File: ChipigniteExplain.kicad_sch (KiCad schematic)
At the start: 73 parts, among them J1 Conn_01x02, J2 Conn_01x02, J3 Conn_01x03, J4 USB_C, J5 613012243121, J6 613012243121, J7 Conn_02x03_Odd_Even, Q1 DMN2005K, SW1 434121025816, SW2 434121025816, SW6 193-8MSR, U1 TLV1117LV33, U2 TPD1E05U06QDPYRQ1, U3 157112V12700

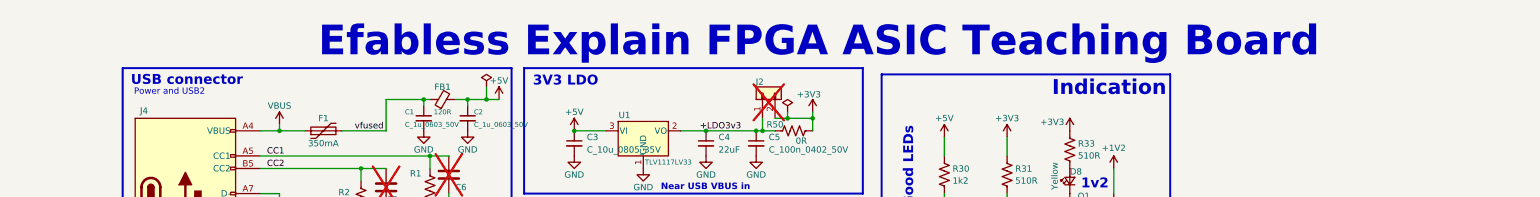
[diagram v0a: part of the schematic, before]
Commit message: title + attrib
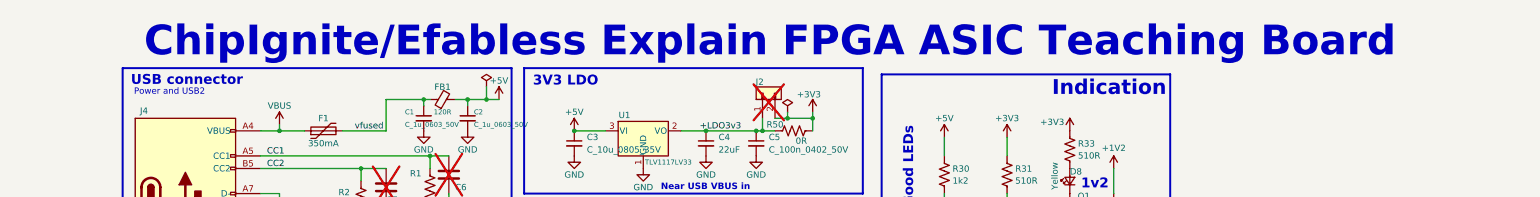
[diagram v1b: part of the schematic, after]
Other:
- note added: "ChipIgnite/Efabless Explain FPGA ASIC Teaching Board"
- note removed: "Efabless Explain FPGA ASIC Teaching Board"
- company: Psychogenic Technologies  -> Psychogenic Technologies for efabless
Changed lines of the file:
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@@
 		(date "2025-02-21")
 		(rev "1.1")
-		(company "Psychogenic Technologies ")
+		(company "Psychogenic Technologies for efabless")
 		(comment 1 "(C) 2024-2025 Pat Deegan")
 	)
@@
 		)
 	)
-	(text "Efabless Explain FPGA ASIC Teaching Board"
+	(text "ChipIgnite/Efabless Explain FPGA ASIC Teaching Board"
 		(exclude_from_sim no)
-		(at 156.21 17.526 0)
+		(at 146.304 17.526 0)
 		(effects
 			(font
